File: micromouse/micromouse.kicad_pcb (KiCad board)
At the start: 2 copper layers, 80 parts, among them IC1 STM32F205RET7, J1 B2B-PH-K-S, J2 B2B-PH-K-S, J3 Left Header, J4 Left Header, Q1 SFH_313_FA-3_4, Q2 SFH_313_FA-3_4, Q3 SFH_313_FA-3_4, Q4 SFH_313_FA-3_4, SW1 CK_KMS2xxG, SW2 EG1218, U1 BS170, U2 AZ1117IH-3.3TRG1, U3 L293DD, U4 BS170, U5 LSM6DSOTR, U6 BS170, U7 BS170

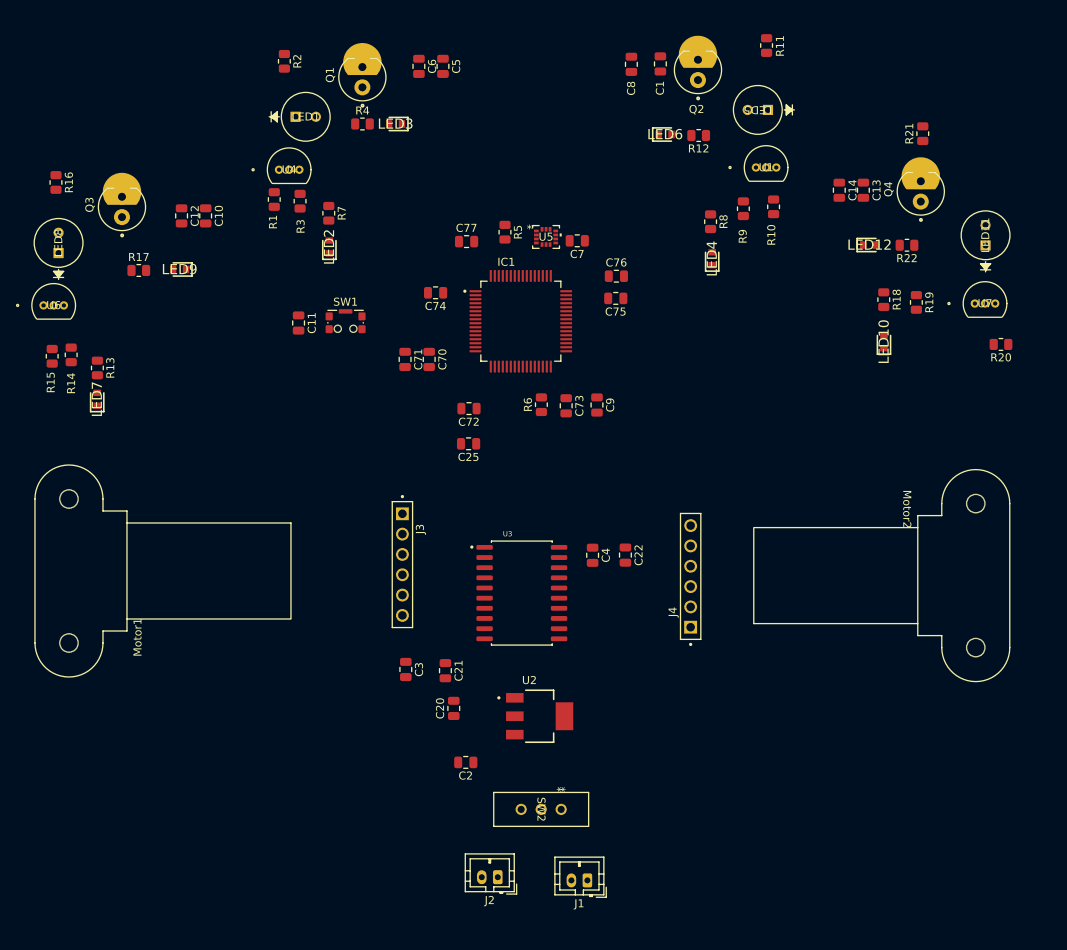
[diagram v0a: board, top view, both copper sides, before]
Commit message: pcb updates
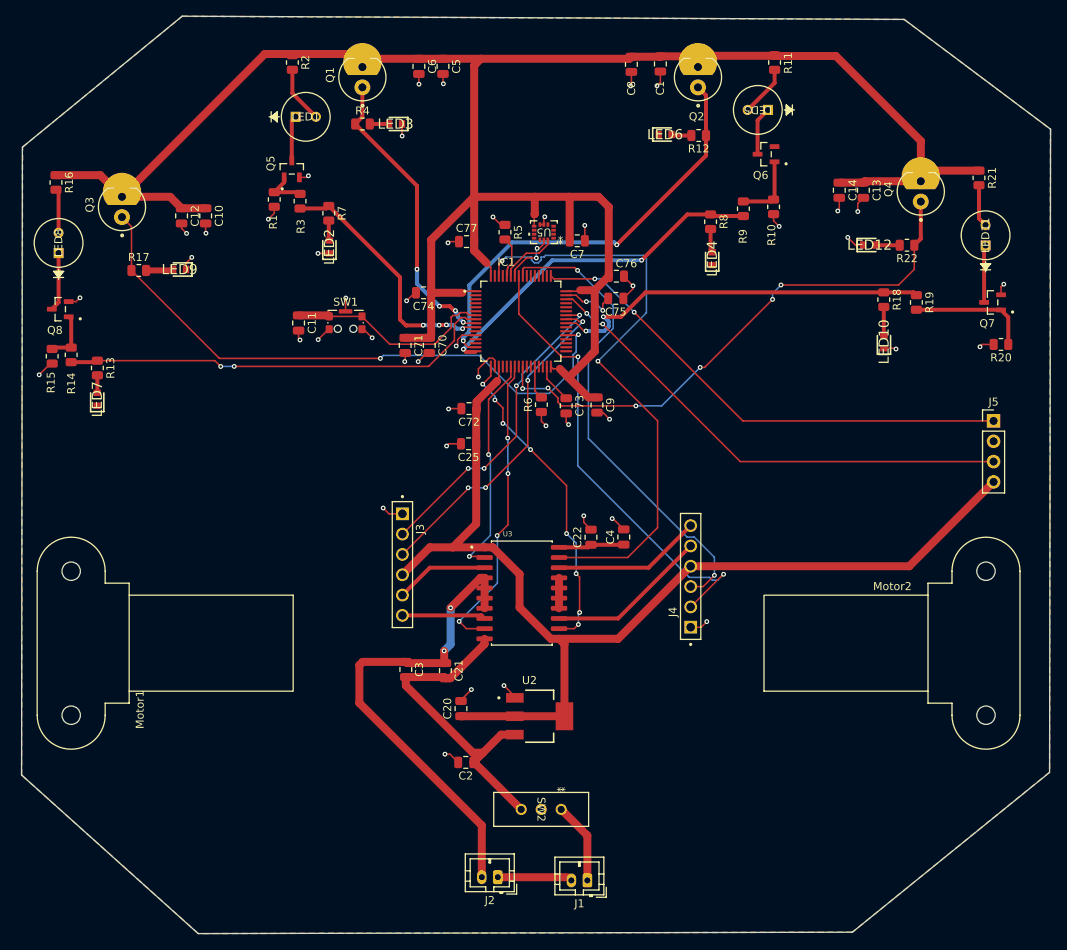
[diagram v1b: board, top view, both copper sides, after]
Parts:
- removed U1, U4, U6, U7: BS170, bs170:TO_SA06_ONS
- added J5: Conn_01x04_Pin, Connector_PinHeader_2.54mm:PinHeader_1x04_P2.54mm_Vertical, F.Cu at (160.7, 61.3)
- added Q5: 2N7002LT1G, new_n_channel_mosfets:SOT95P240X111-3N, F.Cu at (73.0, 29.8)
- added Q6: 2N7002LT1G, new_n_channel_mosfets:SOT95P240X111-3N, F.Cu at (132.3, 28.0)
- added Q7: 2N7002LT1G, new_n_channel_mosfets:SOT95P240X111-3N, F.Cu at (160.6, 46.5)
- added Q8: 2N7002LT1G, new_n_channel_mosfets:SOT95P240X111-3N, F.Cu at (44.1, 47.4)
- moved Motor1 9.03 mm to (48.9, 87.6)
- moved R21 8.94 mm to (158.9, 31.0), turned to -90 degrees
- moved Motor2 8.55 mm to (156.3, 90.6)
- moved C22 4.85 mm to (110.4, 75.9), turned to 90 degrees
- moved C4 4.52 mm to (114.5, 75.8), turned to 90 degrees
- moved R11 2.35 mm to (133.3, 16.5)
- moved C70 1.75 mm to (90.2, 51.9)
- moved C71 1.75 mm to (87.2, 51.9)
- moved C74 1.50 mm to (89.5, 45.3)
- moved R2 1.01 mm to (73.1, 16.5)
- moved Q2 0.91 mm to (123.8, 18.4)
- moved C20 0.90 mm to (94.2, 97.3)
- moved U5 0.66 mm to (104.5, 37.8), turned to 180 degrees
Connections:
- C7 pad 2: +3.3V -> 3V3
- IC1 pad 17: unconnected-(IC1-PA3-Pad17) -> PA3
- IC1 pad 22: unconnected-(IC1-PA6-Pad22) -> PA6
- IC1 pad 23: unconnected-(IC1-PA7-Pad23) -> PA7
- IC1 pad 37: unconnected-(IC1-PC6-Pad37) -> PC6
- IC1 pad 40: unconnected-(IC1-PC9-Pad40) -> PC9
- IC1 pad 41: unconnected-(IC1-PA8-Pad41) -> LENC2
- IC1 pad 42: unconnected-(IC1-PA9-Pad42) -> LENC1
- IC1 pad 56: unconnected-(IC1-PB4-Pad56) -> RENC2
- IC1 pad 57: unconnected-(IC1-PB5-Pad57) -> RENC1
- IC1 pad 62: unconnected-(IC1-PB9-Pad62) -> PB9
- IC1 pad 8: unconnected-(IC1-PC0-Pad8) -> PC0
- J4 pad 3: RENC1 -> RENC2
- Q3 pad 1: PA5 -> PC6
- R13 pad 1: PA6 -> PC0
- R14 pad 1: PA6 -> PC0
- R17 pad 1: PA5 -> PC6
- U3 pad 12: PB8 -> PA3
- U3 pad 2: PB6 -> PA6
- U3 pad 9: PB7 -> PA7
- U5 pad 8: +3.3V -> 3V3
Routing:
- net 3V3: track 0.00 -> 413.2 mm
- net GND: track 0.00 -> 147.8 mm, vias 0 -> 48
- net PC6: track 0.00 -> 76.5 mm, vias 0 -> 2
- net PB9: track 0.00 -> 74.7 mm, vias 0 -> 2
- net PC5: track 0.00 -> 69.3 mm, vias 0 -> 6
- net SWCLK: track 0.00 -> 62.9 mm, vias 0 -> 2
- net SWDIO: track 0.00 -> 61.8 mm, vias 0 -> 2
- net RENC2: track 0.00 -> 59.8 mm, vias 0 -> 2
- net RENC1: track 0.00 -> 58.3 mm, vias 0 -> 2
- net PC0: track 0.00 -> 54.7 mm, vias 0 -> 2
- net PA1: track 0.00 -> 54.7 mm, vias 0 -> 2
- net VCC: track 0.00 -> 49.8 mm
- net PC9: track 0.00 -> 48.0 mm, vias 0 -> 2
- net PA2: track 0.00 -> 43.7 mm, vias 0 -> 2
- net LENC2: track 0.00 -> 41.9 mm, vias 0 -> 4
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- added copper zone on B.Cu, net GND
- added copper zone on F.Cu, net GND
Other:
- board outline added: 128.6 x 114.7 mm
